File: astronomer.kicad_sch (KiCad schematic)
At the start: 46 parts, among them J1 6P6C, SW1 SW_Push_45deg, SW10 SW_Push_45deg, SW11 SW_Push_45deg, SW12 SW_Push_45deg, SW13 SW_Push_45deg, SW14 SW_Push_45deg, SW15 SW_Push_45deg, SW16 SW_Push_45deg, SW17 SW_Push_45deg, SW18 SW_Push_45deg, SW19 SW_Push_45deg, SW2 SW_Push_45deg, SW20 SW_Push_45deg, SW21 SW_Push_45deg, SW22 SW_Push_45deg, SW3 SW_Push_45deg, SW4 SW_Push_45deg, SW5 SW_Push_45deg, SW6 SW_Push_45deg, SW7 SW_Push_45deg, SW8 SW_Push_45deg, SW9 SW_Push_45deg

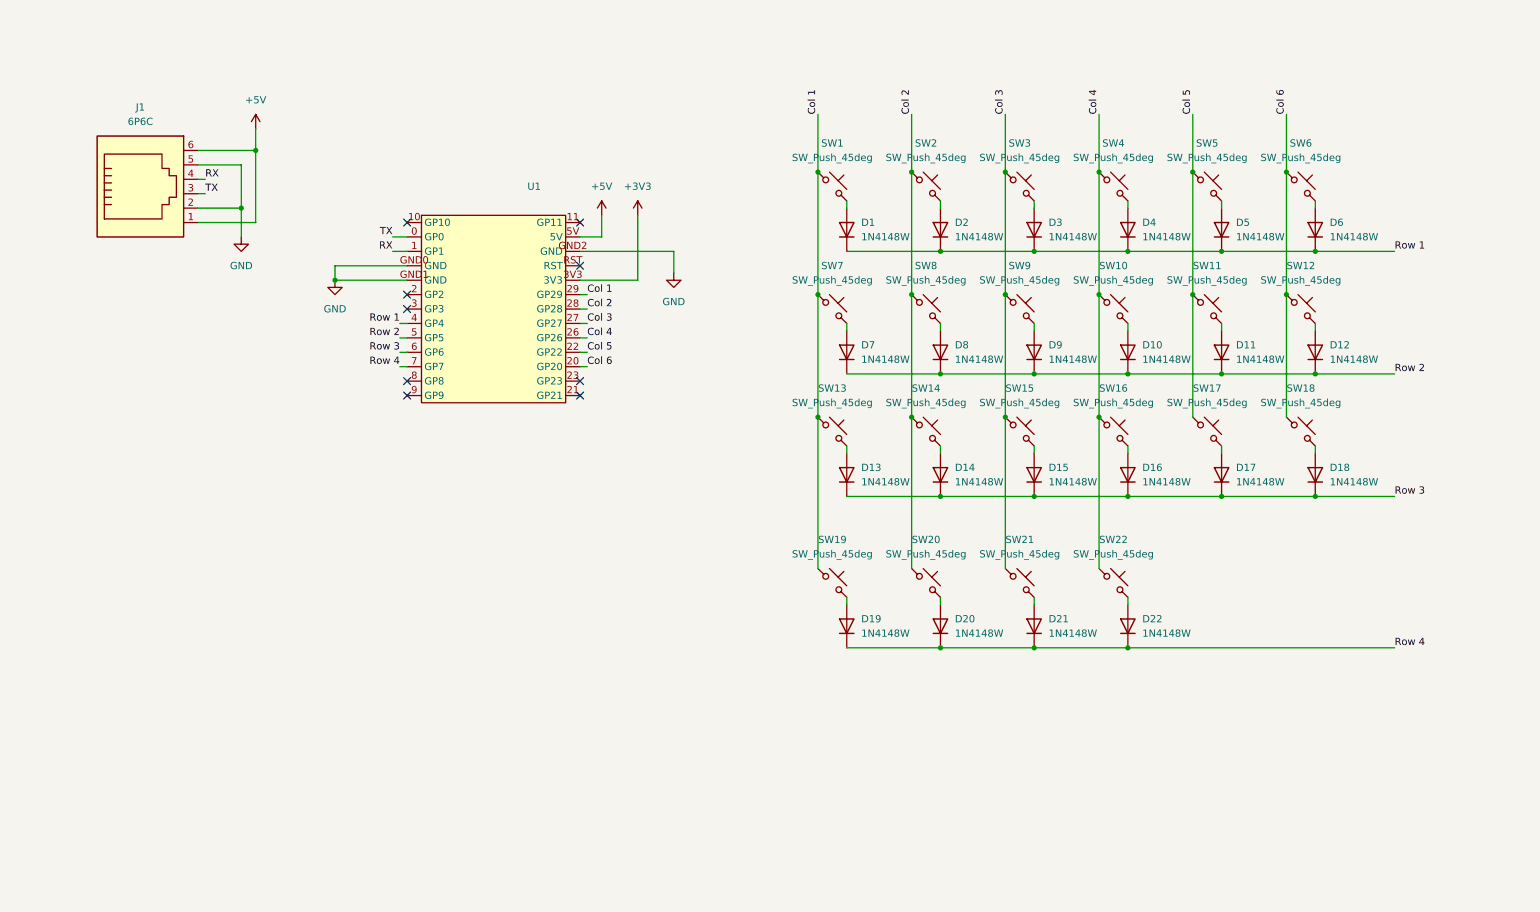
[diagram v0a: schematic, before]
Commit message: lights sch
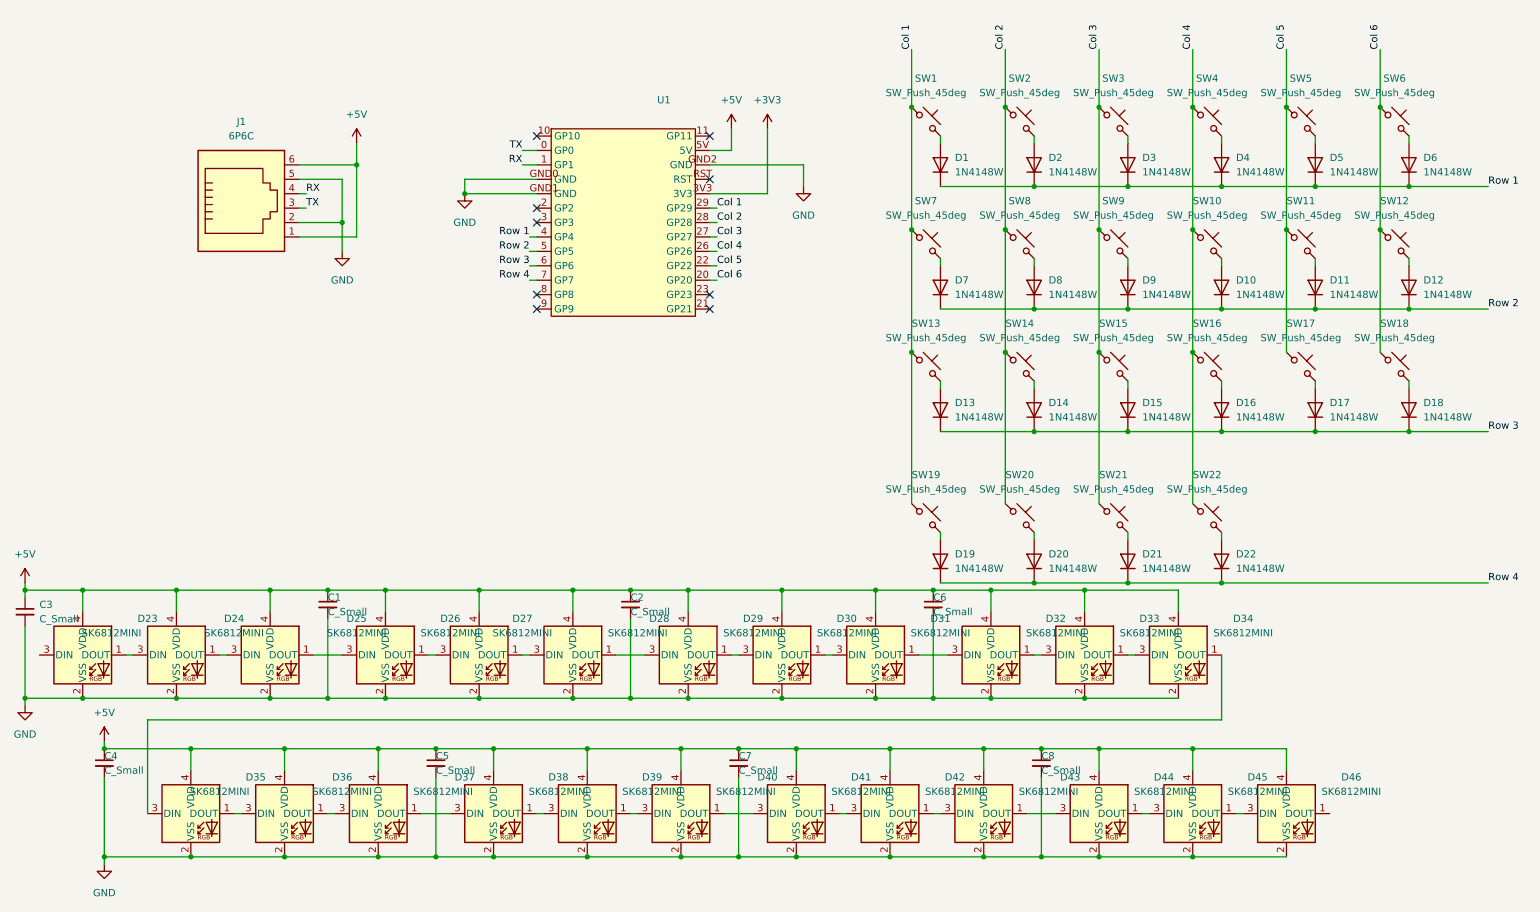
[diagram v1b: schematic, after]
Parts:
- added C1, C2, C3, C4, C5, C6, C7, C8: C_Small, symbol Device:C_Small
- added D23, D24, D25, D26, D27, D28, D29, D30, D31, D32, D33, D34, D35, D36, D37, D38, D39, D40, D41, D42, D43, D44, D45, D46: SK6812MINI, LED_SMD:LED_SK6812MINI_PLCC4_3.5x3.5mm_P1.75mm, symbol LED:SK6812MINI
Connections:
- net +5V: now also C1.1, C2.1, C3.1, C4.1, C5.1, C6.1, C7.1, C8.1, D23.4 (VDD), D24.4 (VDD), D25.4 (VDD), D26.4 (VDD), D27.4 (VDD), D28.4 (VDD), D29.4 (VDD), D30.4 (VDD), D31.4 (VDD), D32.4 (VDD), D33.4 (VDD), D34.4 (VDD), D35.4 (VDD), D36.4 (VDD), D37.4 (VDD), D38.4 (VDD), D39.4 (VDD), D40.4 (VDD), D41.4 (VDD), D42.4 (VDD), D43.4 (VDD), D44.4 (VDD), D45.4 (VDD), D46.4 (VDD)
- net GND: now also C1.2, C2.2, C3.2, C4.2, C5.2, C6.2, C7.2, C8.2, D23.2 (VSS), D24.2 (VSS), D25.2 (VSS), D26.2 (VSS), D27.2 (VSS), D28.2 (VSS), D29.2 (VSS), D30.2 (VSS), D31.2 (VSS), D32.2 (VSS), D33.2 (VSS), D34.2 (VSS), D35.2 (VSS), D36.2 (VSS), D37.2 (VSS), D38.2 (VSS), D39.2 (VSS), D40.2 (VSS), D41.2 (VSS), D42.2 (VSS), D43.2 (VSS), D44.2 (VSS), D45.2 (VSS), D46.2 (VSS)
- new net: D23.1 (DOUT), D24.3 (DIN)
- new net: D25.1 (DOUT), D26.3 (DIN)
- new net: D24.1 (DOUT), D25.3 (DIN)
- new net: D27.1 (DOUT), D28.3 (DIN)
- new net: D26.1 (DOUT), D27.3 (DIN)
- new net: D34.1 (DOUT), D35.3 (DIN)
- new net: D33.1 (DOUT), D34.3 (DIN)
- new net: D30.1 (DOUT), D31.3 (DIN)
- new net: D29.1 (DOUT), D30.3 (DIN)
- new net: D45.1 (DOUT), D46.3 (DIN)
- new net: D44.1 (DOUT), D45.3 (DIN)
- new net: D37.1 (DOUT), D38.3 (DIN)
- new net: D36.1 (DOUT), D37.3 (DIN)
- new net: D39.1 (DOUT), D40.3 (DIN)
- new net: D38.1 (DOUT), D39.3 (DIN)
- new net: D28.1 (DOUT), D29.3 (DIN)
- new net: D32.1 (DOUT), D33.3 (DIN)
- new net: D31.1 (DOUT), D32.3 (DIN)
- new net: D35.1 (DOUT), D36.3 (DIN)
- new net: D43.1 (DOUT), D44.3 (DIN)
- new net: D42.1 (DOUT), D43.3 (DIN)
- new net: D40.1 (DOUT), D41.3 (DIN)
- new net: D41.1 (DOUT), D42.3 (DIN)
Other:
- moved on the sheet: D1, D10, D11, D12, D13, D14, D15, D16, D17, D18, D19, D2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
